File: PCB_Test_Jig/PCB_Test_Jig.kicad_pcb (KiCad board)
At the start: 2 copper layers, 68 x 39.8 mm, 3 parts, among them J1 10018783-10202TLF

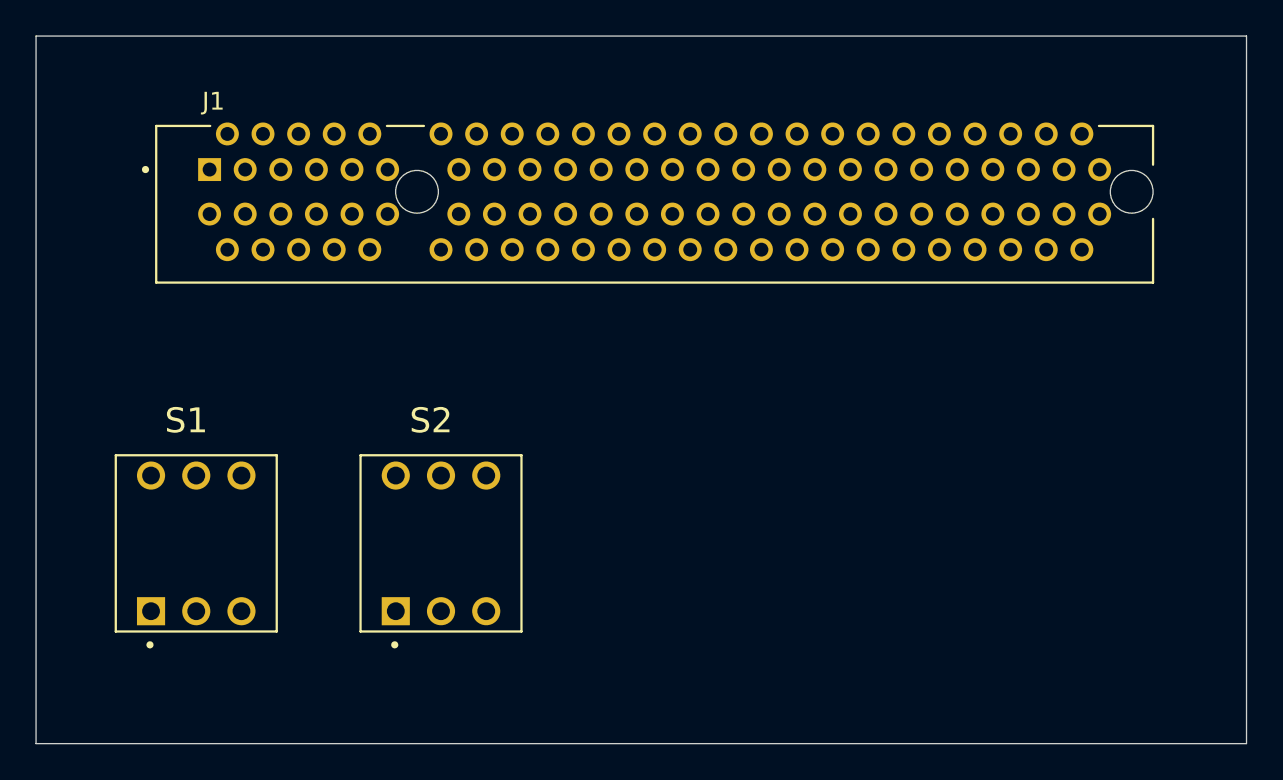
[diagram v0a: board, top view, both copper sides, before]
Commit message: Updated the test jig
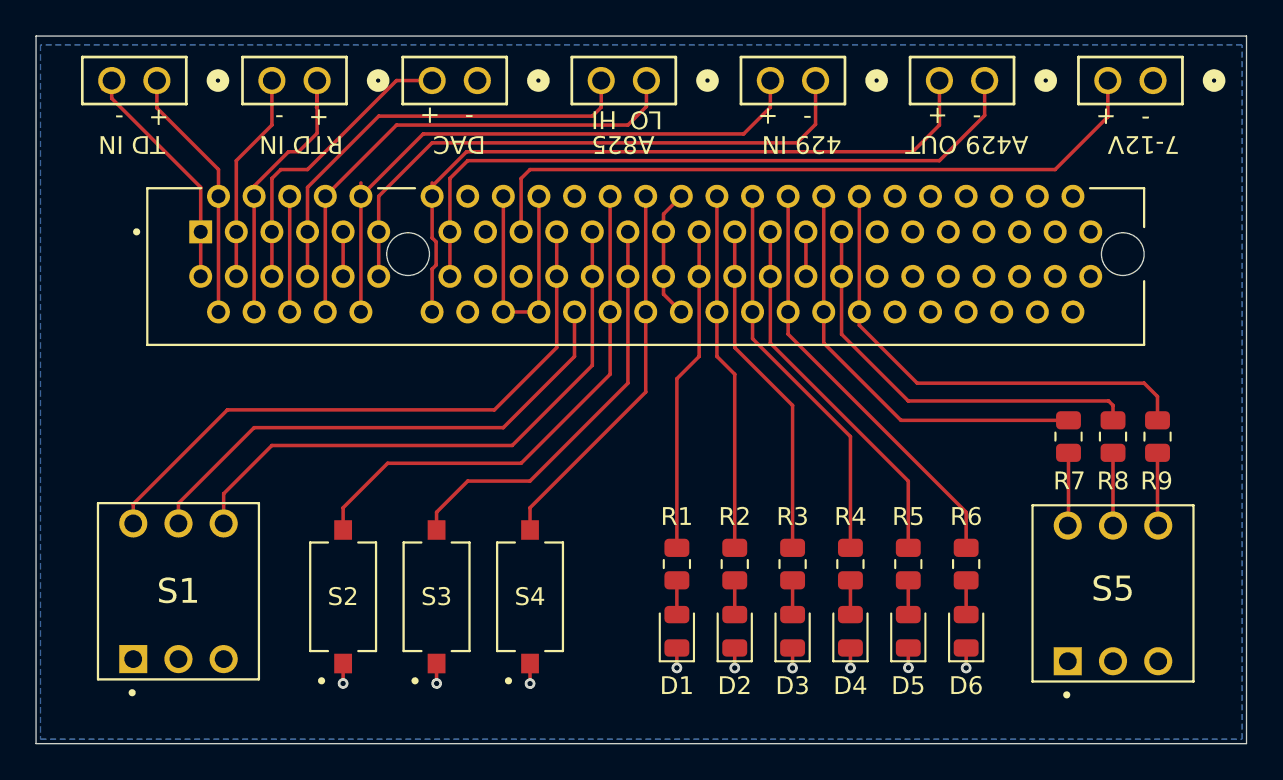
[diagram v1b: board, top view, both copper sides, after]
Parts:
- added D1: LED, LED_SMD:LED_0805_2012Metric, F.Cu at (73.2, 64.4)
- added D2: LED, LED_SMD:LED_0805_2012Metric, F.Cu at (76.5, 64.4)
- added D3: LED, LED_SMD:LED_0805_2012Metric, F.Cu at (79.8, 64.4)
- added D4: LED, LED_SMD:LED_0805_2012Metric, F.Cu at (83.0, 64.4)
- added D5: LED, LED_SMD:LED_0805_2012Metric, F.Cu at (86.2, 64.4)
- added D6: LED, LED_SMD:LED_0805_2012Metric, F.Cu at (89.5, 64.4)
- added G***: LOGO, SDII LIB:Big_Logo, B.Cu at (72.0, 58.5)
- added J2: Conn_01x02_Pin, SDII LIB:pin header, F.Cu at (90.5, 33.5)
- added J3: Conn_01x02_Pin, SDII LIB:pin header, F.Cu at (81.0, 33.5)
- added J4: Conn_01x02_Pin, SDII LIB:pin header, F.Cu at (71.5, 33.5)
- added J5: Conn_01x02_Pin, SDII LIB:pin header, F.Cu at (53.0, 33.5)
- added J6: Conn_01x02_Pin, SDII LIB:pin header, F.Cu at (44.0, 33.5)
- added J7: Conn_01x02_Pin, SDII LIB:pin header, F.Cu at (62.0, 33.5)
- added J8: Conn_01x02_Pin, SDII LIB:pin header, F.Cu at (100.0, 33.5)
- added R1: 1.5k, Resistor_SMD:R_0805_2012Metric, F.Cu at (73.2, 60.7)
- added R2: 1.5k, Resistor_SMD:R_0805_2012Metric, F.Cu at (76.5, 60.7)
- added R3: 1.5k, Resistor_SMD:R_0805_2012Metric, F.Cu at (79.8, 60.7)
- added R4: 1.5k, Resistor_SMD:R_0805_2012Metric, F.Cu at (83.0, 60.7)
- added R5: 1.5k, Resistor_SMD:R_0805_2012Metric, F.Cu at (86.2, 60.7)
- added R6: 1.5k, Resistor_SMD:R_0805_2012Metric, F.Cu at (89.5, 60.7)
- added R7: 1k, Resistor_SMD:R_0805_2012Metric, F.Cu at (95.2, 53.5)
- added R8: 1k, Resistor_SMD:R_0805_2012Metric, F.Cu at (97.8, 53.5)
- added R9: 1k, Resistor_SMD:R_0805_2012Metric, F.Cu at (100.2, 53.5)
- added S2: TS09-63-25-WT-260-SMT-TR, SDII LIB:SW_TS09-63-25-WT-260-SMT-TR, F.Cu at (54.5, 62.5)
- added S3: TS09-63-25-WT-260-SMT-TR, SDII LIB:SW_TS09-63-25-WT-260-SMT-TR, F.Cu at (59.8, 62.5)
- added S4: TS09-63-25-WT-260-SMT-TR, SDII LIB:SW_TS09-63-25-WT-260-SMT-TR, F.Cu at (65.0, 62.5)
- moved S5 51.6 mm to (97.8, 62.3)
- moved S1 15.0 mm to (45.2, 62.2)
- moved J1 3.54 mm to (58.1, 43.2)
- renumbered S2 to S1, S1 to S5
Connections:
- J1 pad A1: unconnected-(J1-PadA1) -> TD-
- J1 pad A10: unconnected-(J1-PadA10) -> A429_IN+
- J1 pad A11: unconnected-(J1-PadA11) -> A429_IN-
- J1 pad A12: unconnected-(J1-PadA12) -> A429_OUT+
- J1 pad A13: unconnected-(J1-PadA13) -> A429_OUT-
- J1 pad A16: unconnected-(J1-PadA16) -> GND
- J1 pad A17: unconnected-(J1-PadA17) -> VCC
- J1 pad A18: unconnected-(J1-PadA18) -> GND
- J1 pad A19: unconnected-(J1-PadA19) -> DSI1
- J1 pad A2: unconnected-(J1-PadA2) -> TD+
- J1 pad A20: unconnected-(J1-PadA20) -> DSI2
- J1 pad A21: unconnected-(J1-PadA21) -> DSI3
- J1 pad A22: unconnected-(J1-PadA22) -> DIS4
- J1 pad A23: unconnected-(J1-PadA23) -> DSI5
- J1 pad A24: unconnected-(J1-PadA24) -> DSI6
- J1 pad A25: unconnected-(J1-PadA25) -> GND
- J1 pad A26: unconnected-(J1-PadA26) -> GND
- J1 pad A27: unconnected-(J1-PadA27) -> DOFB1
- J1 pad A28: unconnected-(J1-PadA28) -> DOFB2
- J1 pad A29: unconnected-(J1-PadA29) -> DOFB3
- J1 pad A3: unconnected-(J1-PadA3) -> RTD-
- J1 pad A30: unconnected-(J1-PadA30) -> DOFB4
- J1 pad A31: unconnected-(J1-PadA31) -> DOFB5
- J1 pad A32: unconnected-(J1-PadA32) -> DOFB6
- J1 pad A33: unconnected-(J1-PadA33) -> GND
- J1 pad A34: unconnected-(J1-PadA34) -> HW_ID_1
- J1 pad A35: unconnected-(J1-PadA35) -> HW_ID_2
- J1 pad A36: unconnected-(J1-PadA36) -> HW_ID_3
- J1 pad A4: unconnected-(J1-PadA4) -> RTD+
- J1 pad A5: unconnected-(J1-PadA5) -> DAC_OUT
- J1 pad A6: unconnected-(J1-PadA6) -> GND
- J1 pad A7: unconnected-(J1-PadA7) -> A825_CAN_HI
- J1 pad A8: unconnected-(J1-PadA8) -> A825_CAN_LO
- J1 pad A9: unconnected-(J1-PadA9) -> GND
- J1 pad B1: unconnected-(J1-PadB1) -> TD-
- J1 pad B10: unconnected-(J1-PadB10) -> A429_IN+
- J1 pad B11: unconnected-(J1-PadB11) -> A429_IN-
- J1 pad B12: unconnected-(J1-PadB12) -> A429_OUT+
- J1 pad B13: unconnected-(J1-PadB13) -> A429_OUT-
- J1 pad B16: unconnected-(J1-PadB16) -> GND
- J1 pad B17: unconnected-(J1-PadB17) -> VCC
- J1 pad B18: unconnected-(J1-PadB18) -> GND
- J1 pad B19: unconnected-(J1-PadB19) -> DSI1
- J1 pad B2: unconnected-(J1-PadB2) -> TD+
- J1 pad B20: unconnected-(J1-PadB20) -> DSI2
- J1 pad B21: unconnected-(J1-PadB21) -> DSI3
- J1 pad B22: unconnected-(J1-PadB22) -> DIS4
- J1 pad B23: unconnected-(J1-PadB23) -> DSI5
- J1 pad B24: unconnected-(J1-PadB24) -> DSI6
- J1 pad B25: unconnected-(J1-PadB25) -> GND
- J1 pad B26: unconnected-(J1-PadB26) -> GND
- J1 pad B27: unconnected-(J1-PadB27) -> DOFB1
- J1 pad B28: unconnected-(J1-PadB28) -> DOFB2
- J1 pad B29: unconnected-(J1-PadB29) -> DOFB3
- J1 pad B3: unconnected-(J1-PadB3) -> RTD-
- J1 pad B30: unconnected-(J1-PadB30) -> DOFB4
- J1 pad B31: unconnected-(J1-PadB31) -> DOFB5
- J1 pad B32: unconnected-(J1-PadB32) -> DOFB6
- J1 pad B33: unconnected-(J1-PadB33) -> GND
- J1 pad B34: unconnected-(J1-PadB34) -> HW_ID_1
- J1 pad B35: unconnected-(J1-PadB35) -> HW_ID_2
- J1 pad B36: unconnected-(J1-PadB36) -> HW_ID_3
- J1 pad B4: unconnected-(J1-PadB4) -> RTD+
- J1 pad B5: unconnected-(J1-PadB5) -> DAC_OUT
- J1 pad B6: unconnected-(J1-PadB6) -> GND
- J1 pad B7: unconnected-(J1-PadB7) -> A825_CAN_HI
- J1 pad B8: unconnected-(J1-PadB8) -> A825_CAN_LO
- J1 pad B9: unconnected-(J1-PadB9) -> GND
- S1 pad 1A: unconnected-(S2-Pad1A) -> GND
- S1 pad 1B: unconnected-(S2-Pad1B) -> DSI1
- S1 pad 2A: unconnected-(S2-Pad2A) -> GND
- S1 pad 2B: unconnected-(S2-Pad2B) -> DSI2
- S1 pad 3A: unconnected-(S2-Pad3A) -> GND
- S1 pad 3B: unconnected-(S2-Pad3B) -> DSI3
- S5 pad 1A: unconnected-(S1-Pad1A) -> GND
- S5 pad 1B: unconnected-(S1-Pad1B) -> Net-(R7-Pad2)
- S5 pad 2A: unconnected-(S1-Pad2A) -> GND
- S5 pad 2B: unconnected-(S1-Pad2B) -> Net-(R8-Pad2)
- S5 pad 3A: unconnected-(S1-Pad3A) -> GND
- S5 pad 3B: unconnected-(S1-Pad3B) -> Net-(R9-Pad2)
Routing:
- net GND: track 0.00 -> 43.9 mm, vias 0 -> 9
- net A429_OUT+: track 0.00 -> 40.4 mm
- net VCC: track 0.00 -> 39.4 mm
- net A429_OUT-: track 0.00 -> 39.0 mm
- net DSI1: track 0.00 -> 35.3 mm
- net A429_IN+: track 0.00 -> 33.8 mm
- net DSI3: track 0.00 -> 33.2 mm
- net A429_IN-: track 0.00 -> 33.2 mm
- net DSI2: track 0.00 -> 29.6 mm
- net DIS4: track 0.00 -> 29.4 mm
- net A825_CAN_LO: track 0.00 -> 28.1 mm
- net HW_ID_3: track 0.00 -> 27.0 mm
- net A825_CAN_HI: track 0.00 -> 24.9 mm
- net DOFB6: track 0.00 -> 23.9 mm
- net HW_ID_1: track 0.00 -> 23.8 mm
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- added copper zone on B.Cu, net GND
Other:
- board text added: "+"
- board text added: "-"
- board text added: "429 IN"
- board text added: "7-12V"
- board text added: "A429 OUT"
- board text added: "A825"
- board text added: "Contributors: Devin Marx"
- board text added: "DAC"
- board text added: "HI"
- board text added: "LO"
- board text added: "RTD IN"
- board text added: "TD IN"
